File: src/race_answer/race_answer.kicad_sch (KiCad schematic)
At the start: 4 parts, among them U1 74LS175, U2 74LS148, U3 74LS20, U4 74LS00

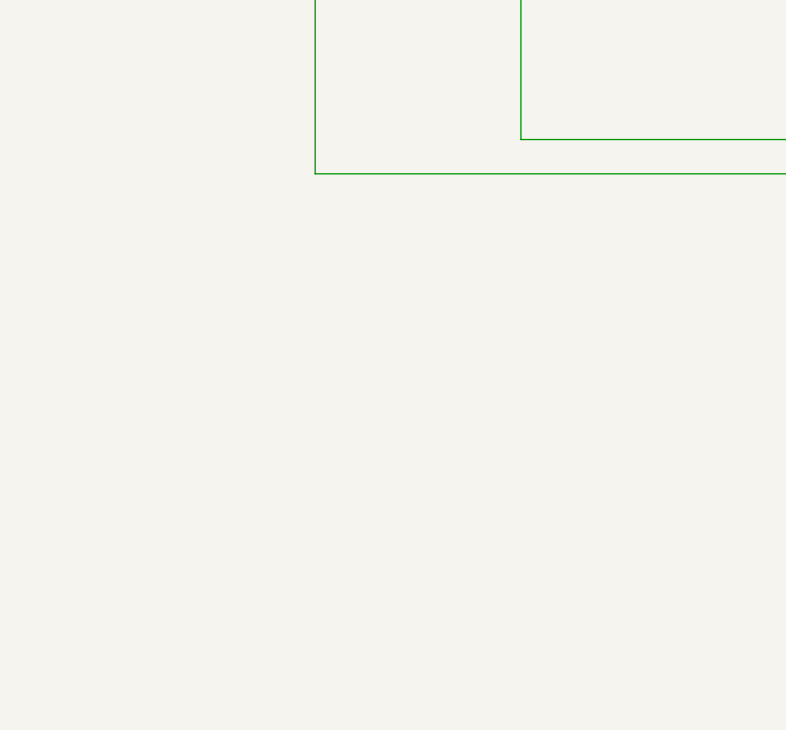
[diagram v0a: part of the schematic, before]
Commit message: race-answer
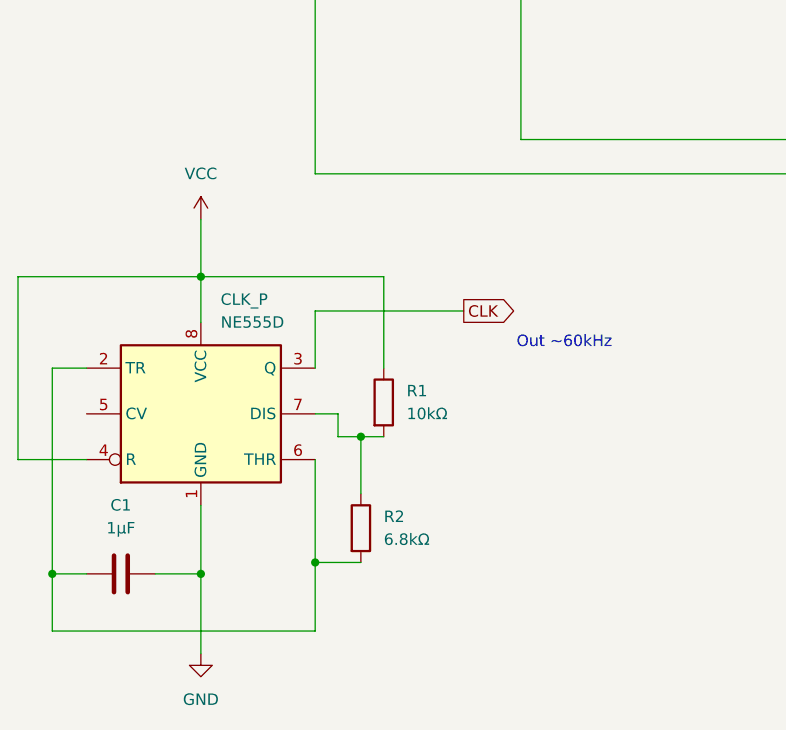
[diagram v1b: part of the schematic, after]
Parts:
- added C1: 1μF, symbol Device:C
- added CLK_P: NE555D, Package_SO:SOIC-8_3.9x4.9mm_P1.27mm, symbol Timer:NE555D
- added R1: 10kΩ, symbol Device:R
- added R2: 6.8kΩ, symbol Device:R
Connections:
- net CLK: now also CLK_P.3 (Q)
- net GND: now also C1.2, CLK_P.1 (GND)
- net VCC: now also CLK_P.4 (R), CLK_P.8 (VCC), R1.1
- new net: CLK_P.7 (DIS), R1.2, R2.1
- new net: C1.1, CLK_P.2 (TR), CLK_P.6 (THR), R2.2
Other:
- note added: "Out ~60kHz"
